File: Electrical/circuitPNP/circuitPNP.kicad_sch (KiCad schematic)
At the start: 8 parts, among them Q1 GS66504B, Q2 GS66504B, U1 ESP32-S3-WROOM-1, U2 STMPE1600

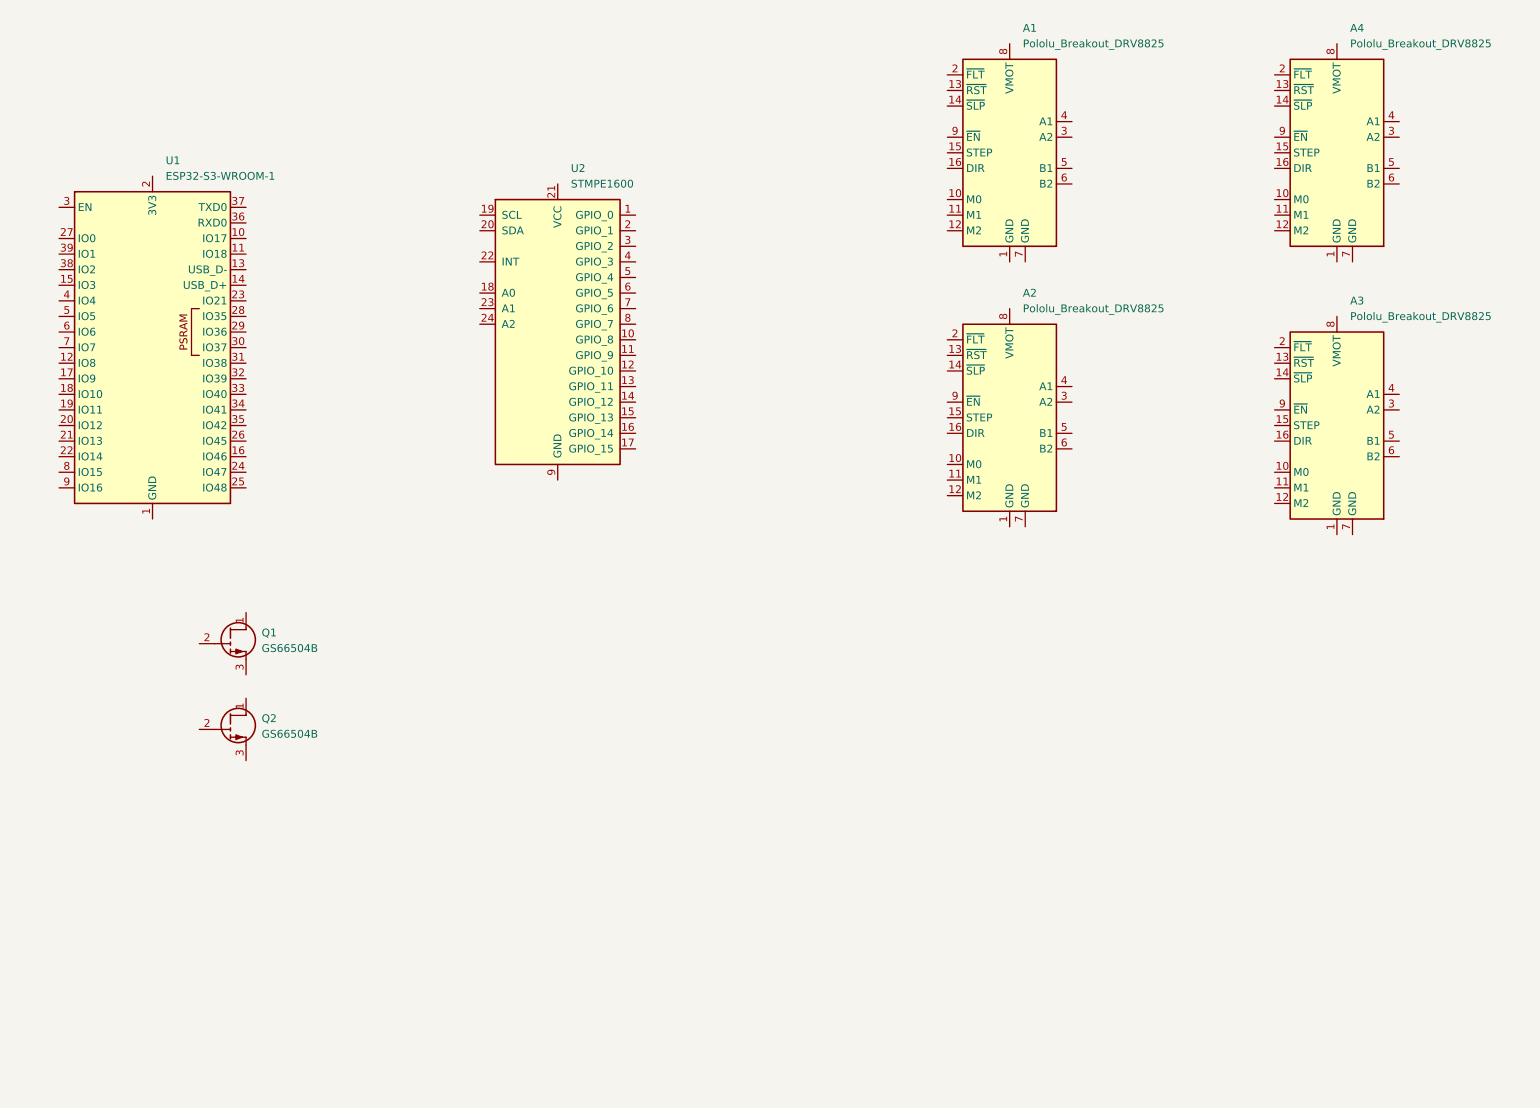
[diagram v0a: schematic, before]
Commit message: wip and gitignore update
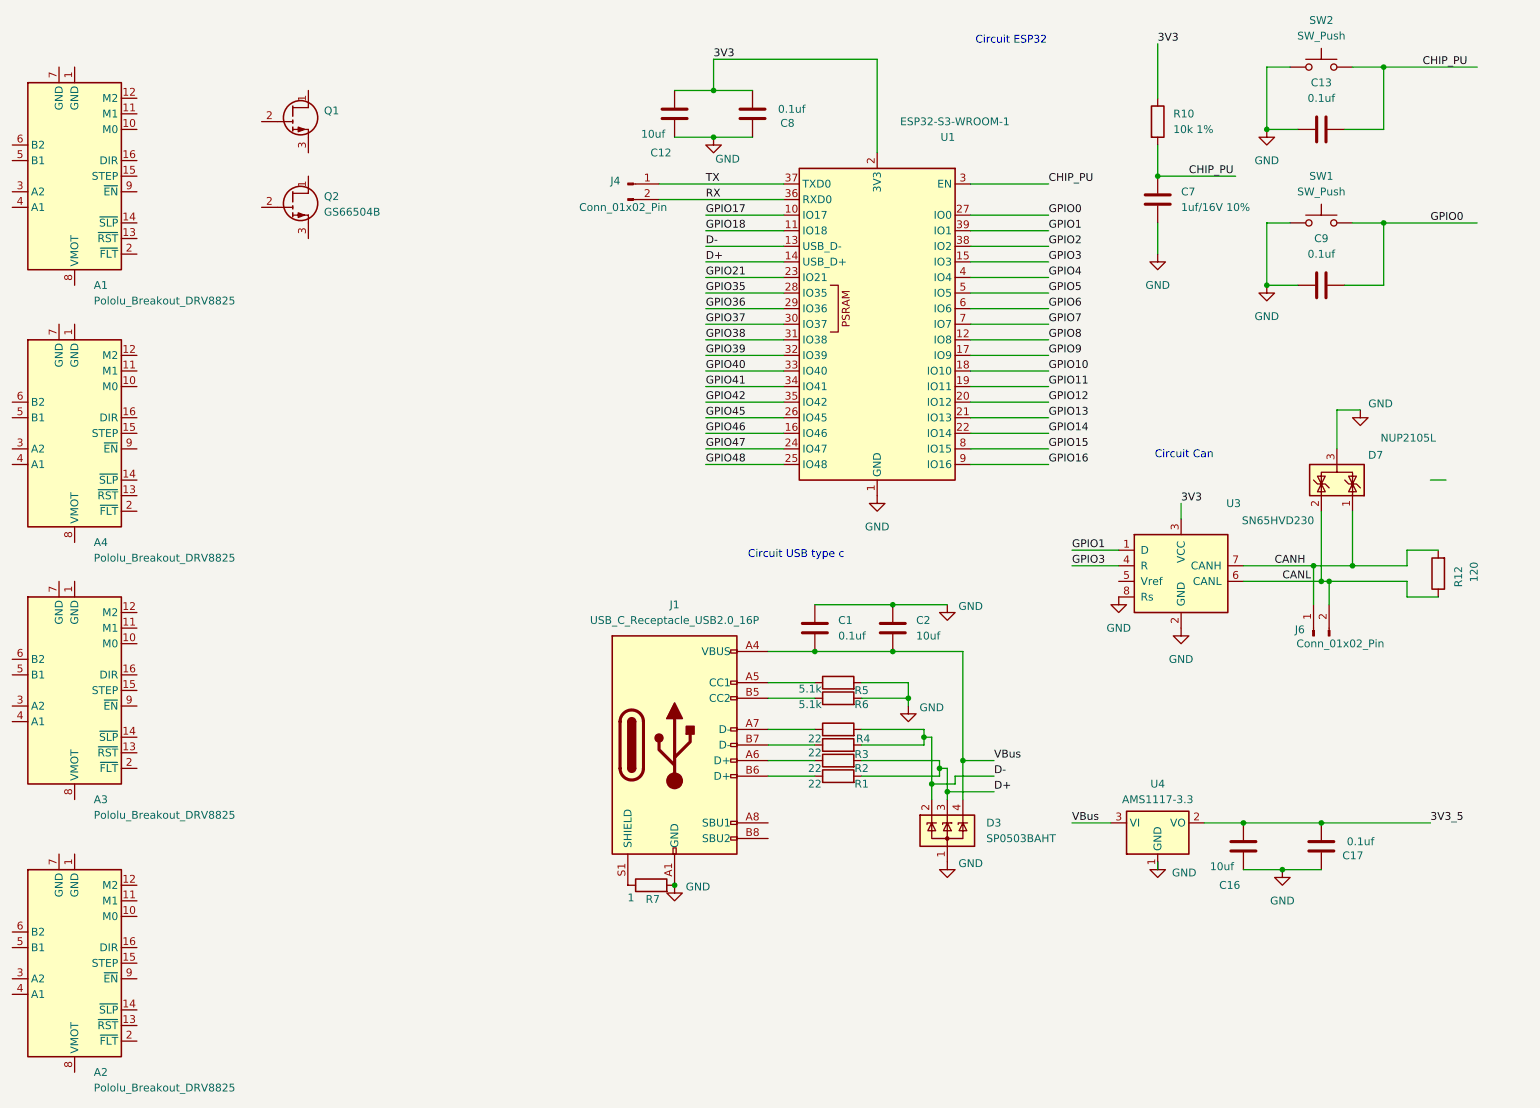
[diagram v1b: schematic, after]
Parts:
- removed U2: STMPE1600, Package_DFN_QFN:QFN-24-1EP_4x4mm_P0.5mm_EP2.6x2.6mm, symbol Interface_Expansion:STMPE1600
- added C1, C13, C17, C8, C9: 0.1uf, Capacitor_SMD:C_0603_1608Metric_Pad1.08x0.95mm_HandSolder, symbol Device:C
- added C12, C16, C2: 10uf, Capacitor_SMD:C_0603_1608Metric_Pad1.08x0.95mm_HandSolder, symbol Device:C
- added C7: 1uf/16V 10%, Capacitor_SMD:C_0603_1608Metric_Pad1.08x0.95mm_HandSolder, symbol Device:C
- added D3: SP0503BAHT, Package_TO_SOT_SMD:SOT-143, symbol Power_Protection:SP0503BAHT
- added D7: NUP2105L, Package_TO_SOT_SMD:SOT-23, symbol Power_Protection:NUP2105L
- added J1: USB_C_Receptacle_USB2.0_16P, Connector_USB:USB_C_Receptacle_GCT_USB4105-xx-A_16P_TopMnt_Horizontal, symbol Connector:USB_C_Receptacle_USB2.0_16P
- added J4: Conn_01x02_Pin, Connector_PinHeader_2.54mm:PinHeader_1x02_P2.54mm_Vertical, symbol Connector:Conn_01x02_Pin
- added J6: Conn_01x02_Pin, Connector_Molex:Molex_KK-396_A-41792-0002_1x02_P3.96mm_Horizontal, symbol Connector:Conn_01x02_Pin
- added R1, R2, R3, R4: 22, Resistor_SMD:R_0603_1608Metric_Pad0.98x0.95mm_HandSolder, symbol Device:R
- added R10: 10k 1%, Resistor_SMD:R_0603_1608Metric_Pad0.98x0.95mm_HandSolder, symbol Device:R
- added R12: 120, Resistor_SMD:R_0603_1608Metric_Pad0.98x0.95mm_HandSolder, symbol Device:R
- added R5, R6: 5.1k, Resistor_SMD:R_0603_1608Metric_Pad0.98x0.95mm_HandSolder, symbol Device:R
- added R7: 1, Resistor_SMD:R_0603_1608Metric_Pad0.98x0.95mm_HandSolder, symbol Device:R
- added SW1, SW2: SW_Push, Button_Switch_SMD:SW_SPST_PTS647_Sx38, symbol Switch:SW_Push
- added U3: SN65HVD230, Package_SO:SOIC-8_3.9x4.9mm_P1.27mm, symbol Interface_CAN_LIN:SN65HVD230
- added U4: AMS1117-3.3, Package_TO_SOT_SMD:SOT-223-3_TabPin2, symbol Regulator_Linear:AMS1117-3.3
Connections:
- net GND: now reaches U1.1 (GND), U1.40 (GND), U1.41 (GND)
- net GND: now also C1.1, C12.1, C13.2, C16.1, C17.1, C2.1, C7.2, C8.1, C9.2, D3.1 (A), D7.3 (A), J1.A1 (GND), J1.A12 (GND), J1.B1 (GND), J1.B12 (GND), R5.2, R6.2, R7.2, SW1.1, SW2.1, U3.2 (GND), U3.8 (Rs), U4.1 (GND)
- net GPIO17: now reaches U1.10 (IO17)
- net GPIO18: now reaches U1.11 (IO18)
- net GPIO8: now reaches U1.12 (IO8)
- net D-: now reaches U1.13 (USB_D-)
- net D-: now also D3.2 (K), R3.2, R4.2
- net D+: now reaches U1.14 (USB_D+)
- net D+: now also D3.3 (K), R1.2, R2.2
- net GPIO3: now reaches U1.15 (IO3)
- net GPIO3: now also U3.4 (R)
- net GPIO46: now reaches U1.16 (IO46)
- net GPIO9: now reaches U1.17 (IO9)
- net GPIO10: now reaches U1.18 (IO10)
- net GPIO11: now reaches U1.19 (IO11)
- net 3V3: now reaches U1.2 (3V3)
- net 3V3: now also C12.2, C8.2, R10.1, U3.3 (VCC)
- net GPIO12: now reaches U1.20 (IO12)
- net GPIO13: now reaches U1.21 (IO13)
- net GPIO14: now reaches U1.22 (IO14)
- net GPIO21: now reaches U1.23 (IO21)
- net GPIO47: now reaches U1.24 (IO47)
- net GPIO48: now reaches U1.25 (IO48)
- net GPIO45: now reaches U1.26 (IO45)
- net GPIO0: now reaches U1.27 (IO0)
- net GPIO0: now also C9.1, SW1.2
- net GPIO35: now reaches U1.28 (IO35)
- net GPIO36: now reaches U1.29 (IO36)
- net CHIP_PU: now reaches U1.3 (EN)
- net CHIP_PU: now also C13.1, C7.1, R10.2, SW2.2
- net GPIO37: now reaches U1.30 (IO37)
- net GPIO38: now reaches U1.31 (IO38)
- net GPIO39: now reaches U1.32 (IO39)
- net GPIO40: now reaches U1.33 (IO40)
- net GPIO41: now reaches U1.34 (IO41)
- net GPIO42: now reaches U1.35 (IO42)
- net RX: now reaches U1.36 (RXD0)
- net RX: now also J4.2 (Pin_2)
- net TX: now reaches U1.37 (TXD0)
- net TX: now also J4.1 (Pin_1)
- net GPIO2: now reaches U1.38 (IO2)
- net GPIO1: now reaches U1.39 (IO1)
- net GPIO1: now also U3.1 (D)
- net GPIO4: now reaches U1.4 (IO4)
- net GPIO5: now reaches U1.5 (IO5)
- net GPIO6: now reaches U1.6 (IO6)
- net GPIO7: now reaches U1.7 (IO7)
- net GPIO15: now reaches U1.8 (IO15)
- net GPIO16: now reaches U1.9 (IO16)
- new net: J1.S1 (SHIELD), R7.1
- new net: J1.B5 (CC2), R6.1
- new net: J1.B6 (D+), R1.1
- new net: J1.B7 (D-), R3.1
- new net: J1.A7 (D-), R4.1
- new net: J1.A5 (CC1), R5.1
- new net: J1.A6 (D+), R2.1
- new net 3V3_5: C16.2, C17.2, U4.2 (VO)
- new net CANH: D7.1 (K), J6.1 (Pin_1), R12.2, U3.7 (CANH)
- new net CANL: D7.2 (K), J6.2 (Pin_2), R12.1, U3.6 (CANL)
- new net VBus: C1.2, C2.2, D3.4 (K), J1.A4 (VBUS), J1.A9 (VBUS), J1.B4 (VBUS), J1.B9 (VBUS), U4.3 (VI)
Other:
- note added: "Circuit Can"
- note added: "Circuit ESP32"
- note added: "Circuit USB type c"
- moved on the sheet: A1, A2, A3, A4, Q1, Q2
